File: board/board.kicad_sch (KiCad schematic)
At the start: 1 part

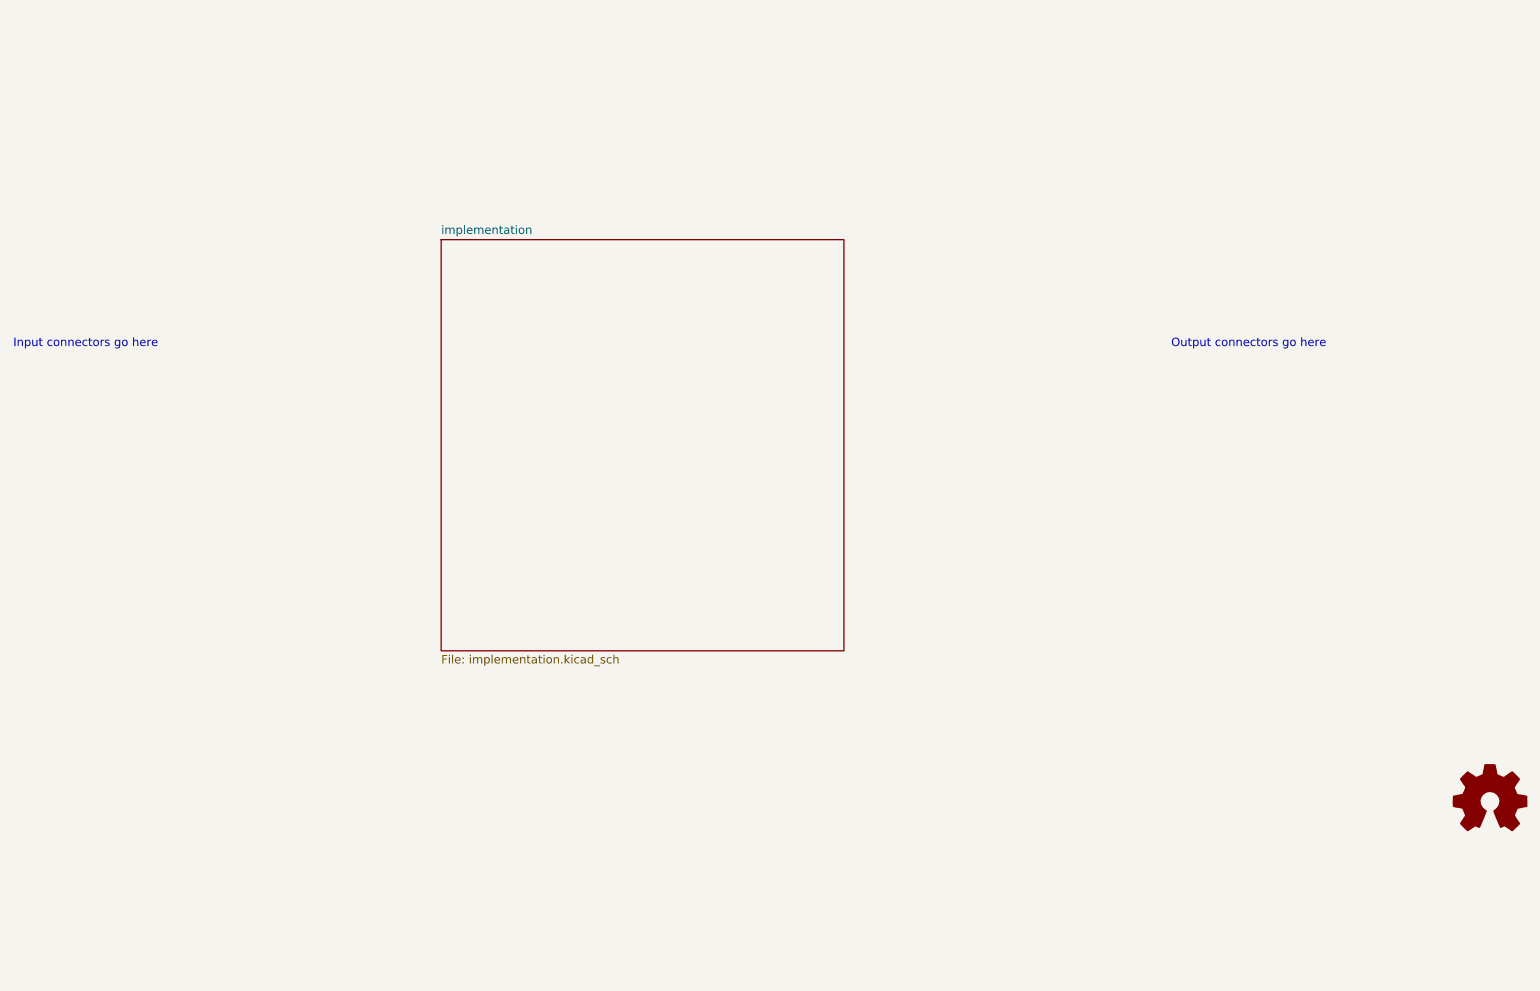
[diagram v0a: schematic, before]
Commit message: imported legacy version
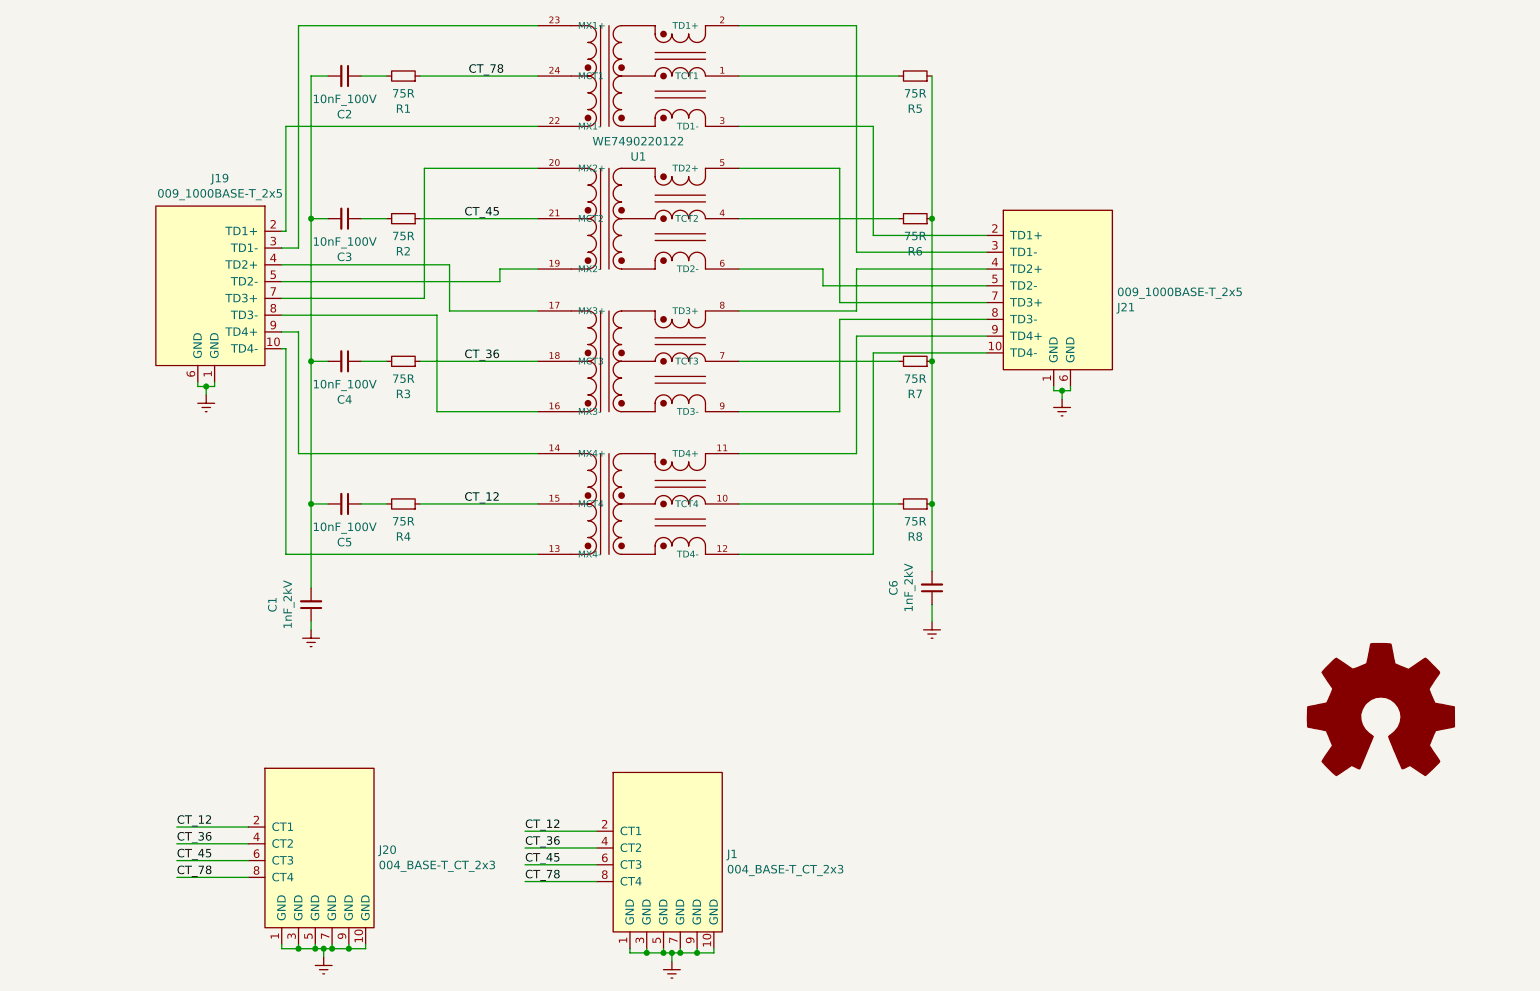
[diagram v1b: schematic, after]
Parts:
- removed LOGO1: Logo_Open_Hardware_Small, Symbol:OSHW-Symbol_6.7x6mm_SilkScreen, symbol Graphic:Logo_Open_Hardware_Small
- added C1, C6: 1nF_2kV, Capacitor_SMD:C_1210_3225Metric, symbol Device:C_Small
- added C2, C3, C4, C5: 10nF_100V, Capacitor_SMD:C_0603_1608Metric, symbol Device:C_Small
- added J1: 004_BASE-T_CT_2x3, on_edge:on_edge_2x05_device, symbol put_on_edge:004_BASE-T_CT
- added J19, J21: 009_1000BASE-T_2x5, on_edge:on_edge_2x05_host, symbol put_on_edge:009_1000BASE-T
- added J20: 004_BASE-T_CT_2x3, on_edge:on_edge_2x05_host, symbol put_on_edge:004_BASE-T_CT
- added R1, R2, R3, R4, R5, R6, R7, R8: 75R, Resistor_SMD:R_0805_2012Metric, symbol Device:R_Small
- added U1: WE7490220122, AI-footprints:XFMR_7490220122, symbol Auto-Intern:WE7490220122
- added l1: Logo_Open_Hardware_Large, Symbol:OSHW-Logo2_7.3x6mm_SilkScreen, symbol Graphic:Logo_Open_Hardware_Large
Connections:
- new net: C5.1, R4.2
- new net: C1.2, C2.2, C3.2, C4.2, C5.2
- new net: C6.2, R5.1, R6.1, R7.1, R8.1
- new net: R8.2, U1.10 (TCT4)
- new net: R7.2, U1.7 (TCT3)
- new net: R6.2, U1.4 (TCT2)
- new net: R5.2, U1.1 (TCT1)
- new net: C4.1, R3.2
- new net: C3.1, R2.2
- new net: C2.1, R1.2
- new net: J21.9 (TD4+), U1.11 (TD4+)
- new net: J21.10 (TD4-), U1.12 (TD4-)
- new net: J19.10 (TD4-), U1.13 (MX4-)
- new net: J19.9 (TD4+), U1.14 (MX4+)
- new net: J19.8 (TD3-), U1.16 (MX3-)
- new net: J19.4 (TD2+), U1.17 (MX3+)
- new net: J19.5 (TD2-), U1.19 (MX2-)
- new net: J21.3 (TD1-), U1.2 (TD1+)
- new net: J19.7 (TD3+), U1.20 (MX2+)
- new net: J19.2 (TD1+), U1.22 (MX1-)
- new net: J19.3 (TD1-), U1.23 (MX1+)
- new net: J21.2 (TD1+), U1.3 (TD1-)
- new net: J21.7 (TD3+), U1.5 (TD2+)
- new net: J21.5 (TD2-), U1.6 (TD2-)
- new net: J21.4 (TD2+), U1.8 (TD3+)
- new net: J21.8 (TD3-), U1.9 (TD3-)
- new net CT_12: J1.2 (CT1), J20.2 (CT1), R4.1, U1.15 (MCT4)
- new net CT_36: J1.4 (CT2), J20.4 (CT2), R3.1, U1.18 (MCT3)
- new net CT_45: J1.6 (CT3), J20.6 (CT3), R2.1, U1.21 (MCT2)
- new net CT_78: J1.8 (CT4), J20.8 (CT4), R1.1, U1.24 (MCT1)
- new net Earth: C1.1, C6.1, J1.1 (GND), J1.10 (GND), J1.3 (GND), J1.5 (GND), J1.7 (GND), J1.9 (GND), J19.1 (GND), J19.6 (GND), J20.1 (GND), J20.10 (GND), J20.3 (GND), J20.5 (GND), J20.7 (GND), J20.9 (GND), J21.1 (GND), J21.6 (GND)
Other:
- removed sheet implementation
- note removed: "Input connectors go here"
- note removed: "Output connectors go here"
